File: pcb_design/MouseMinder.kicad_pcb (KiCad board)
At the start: 2 copper layers, 25.5 x 40.7 mm, 24 parts, among them J3 Conn_02x04_Odd_Even, SW1 LCK-TA022H18-2WL, SW2 SKRPABE010, U1 PMS150C

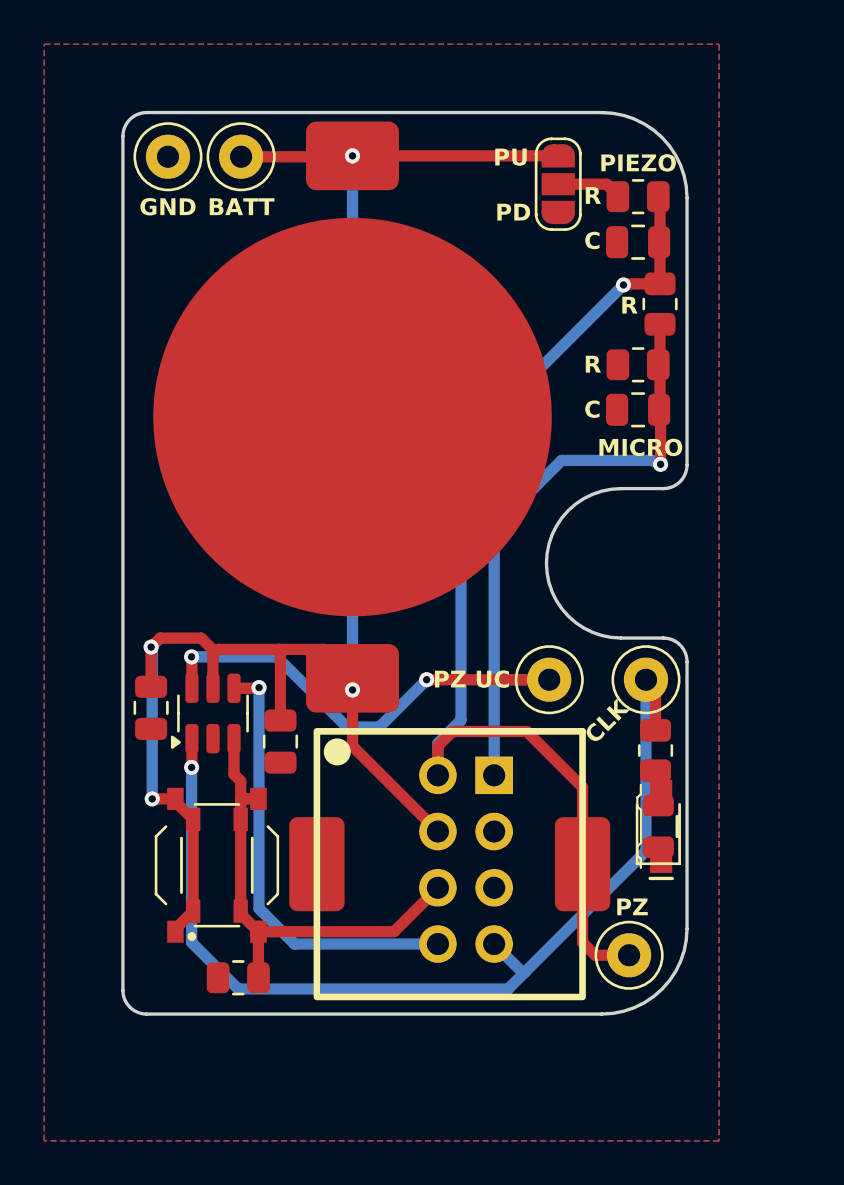
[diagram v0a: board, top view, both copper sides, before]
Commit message: R6 sent to JLC Today. Here is the full prod snapshot.
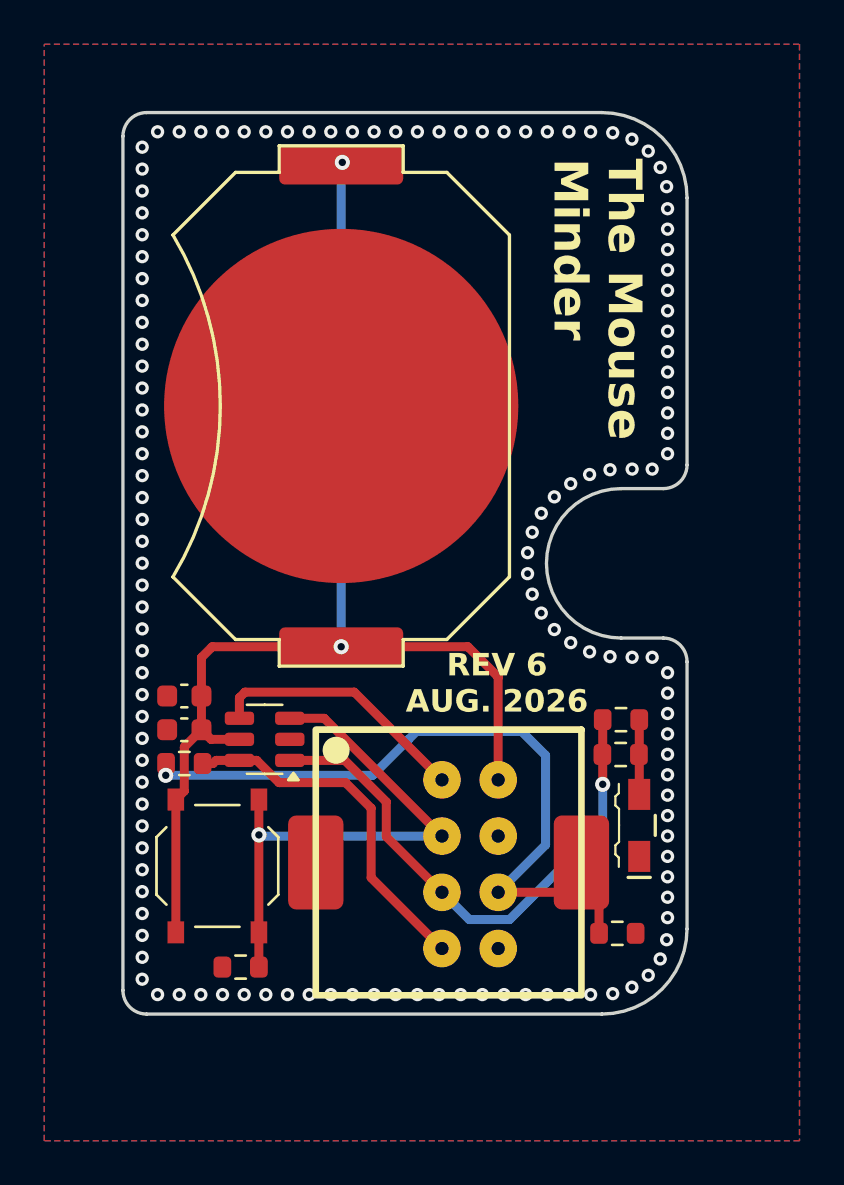
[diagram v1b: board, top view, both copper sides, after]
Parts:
- removed C1, C2: 1u, Capacitor_SMD:C_0805_2012Metric
- removed D2: LED, LED_SMD:LED_0805_2012Metric
- removed the G*** at (-25.9, 8.36)
- removed JP1: SolderJumper_3_Open, Jumper:SolderJumper-3_P1.3mm_Open_RoundedPad1.0x1.5mm_NumberLabels
- removed R5: 100, Resistor_SMD:R_0805_2012Metric
- removed SW2: SKRPABE010, 0conrads:SKRPABE010
- removed TP1, TP2, TP3, TP4, TP5: TestPoint, TestPoint:TestPoint_Loop_D2.50mm_Drill1.0mm
- added G***: LOGO, 0art:POGO, B.Cu at (-20.1, 15.2)
- added R6: 100, Resistor_SMD:R_0603_1608Metric, F.Cu at (-13.3, 20.7)
- BT1: footprint 0conrads:C70373 -> 0conrads:MY-2032-08
- C3, C4: footprint Capacitor_SMD:C_0805_2012Metric -> Capacitor_SMD:C_0603_1608Metric
- J3: footprint Connector_PinHeader_2.54mm:PinHeader_2x04_P2.54mm_Vertical -> 0conrads:2x8_POGO_CENTERING_HOLES
- R1, R2, R3, R4: footprint Resistor_SMD:R_0805_2012Metric -> Resistor_SMD:R_0603_1608Metric
- moved R1 33.3 mm to (-13.5, 28.7), turned to 180 degrees
- moved R2 29.9 mm to (-33.0, 21.1), turned to 180 degrees
- moved C3 4.38 mm to (-33.0, 19.5), turned to 180 degrees
- moved U1 2.61 mm to (-29.4, 20.0), turned to 180 degrees
- moved R3 2.09 mm to (-13.3, 19.1), turned to 0 degrees
- moved C4 1.59 mm to (-33.0, 18.0), turned to 180 degrees
- moved D1 0.99 mm to (-12.6, 23.9)
- moved BT1 0.72 mm to (-26.0, 4.91)
- moved R4 0.49 mm to (-30.5, 30.3)
- moved J3 0.27 mm to (-18.9, 21.8)
- moved BZ1 0.09 mm to (-21.1, 25.5)
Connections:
- J3 pad 1: PIEZO_UC -> +3V0
- J3 pad 2: PIEZO -> HVPROG
- J3 pad 3: GND -> unconnected-(J3-Pin_3-Pad3)
- J3 pad 4: +3V0 -> PROGMODE
- J3 pad 5: unconnected-(J3-Pin_5-Pad5) -> PIEZO
- J3 pad 6: PROGMODE -> CLK
- J3 pad 7: CLK -> GND
- J3 pad 8: HVPROG -> PIEZO_UC
- R1 pad 1: Net-(JP1-C) -> GND
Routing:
- net PIEZO_UC: track 48.7 -> 16.2 mm, vias 3 -> 0
- net +3V0: track 79.0 -> 55.6 mm, vias 4 -> 2
- net CLK: track 45.3 -> 24.6 mm
- net PIEZO: track 50.5 -> 34.4 mm
- net HVPROG: track 19.9 -> 11.8 mm, vias 1 -> 0
- net PROGMODE: track 21.0 -> 24.9 mm, vias 0 -> 1
- net Net-(D1-A): track 0.00 -> 3.38 mm
- net Net-(JP1-C): track 2.98 -> 0.00 mm
- net GND: vias 0 -> 135
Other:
- board text added: "DAT"
- board text added: "REV 6 AUG. 2026"
- board text added: "ROHS"
- board text added: "The Mouse Minder"
- board text removed: "BATT"
- board text removed: "C"
- board text removed: "MICRO"
- board text removed: "PD"
- board text removed: "PIEZO"
- board text removed: "PU"
- board text removed: "PZ UC"
- board text removed: "R"
- board text removed: "REVISION 5 JUL. 2026"
- board text removed: "TO DO: Fix Pogo Programmer Holes!"
